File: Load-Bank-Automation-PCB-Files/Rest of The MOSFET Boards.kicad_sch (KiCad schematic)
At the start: 17 parts, among them J25 Conn_02x03_Counter_Clockwise, J27 PHNX_CONN_1017521, Q4 GSGN0648, U11 IRS10752LPBF, U9 ACS711xLCTR-25AB

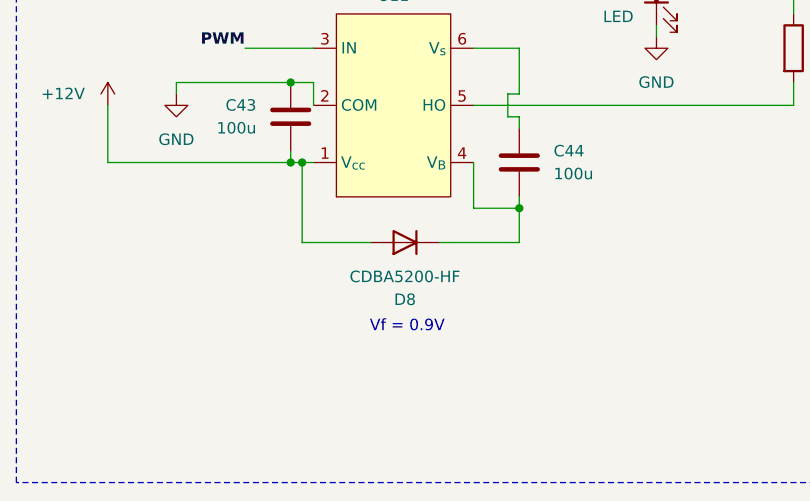
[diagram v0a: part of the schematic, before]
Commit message: Schematic for revision
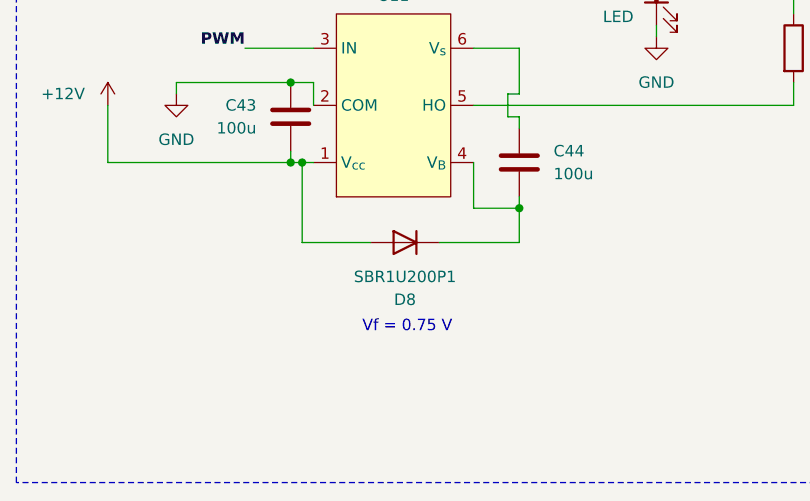
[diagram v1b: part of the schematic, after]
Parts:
- D8: value CDBA5200-HF -> SBR1U200P1; footprint Diode_SMD:D_SMA -> Diode_SMD:D_PowerDI-123
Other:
- note added: "Vf = 0.75 V"
- note removed: "Vf = 0.9V"
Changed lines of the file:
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@@
 		)
 	)
-	(text "Vf = 0.9V\n"
+	(text "Vf = 0.75 V\n"
 		(exclude_from_sim no)
 		(at 76.454 144.018 0)
@@
 	)
 	(symbol
+		(lib_id "Device:D")
+		(at 76.2 134.62 0)
+		(mirror y)
+		(unit 1)
+		(exclude_from_sim no)
+		(in_bom yes)
+		(on_board yes)
+		(dnp no)
+		(property "Reference" "D8"
+			(at 76.2 140.97 0)
+			(effects
+				(font
+					(size 1.27 1.27)
+				)
+			)
+		)
+		(property "Value" "SBR1U200P1"
+			(at 76.2 138.43 0)
+			(effects
+				(font
+					(size 1.27 1.27)
+				)
+			)
+		)
+		(property "Footprint" "Diode_SMD:D_PowerDI-123"
+			(at 76.2 134.62 0)
+			(effects
+				(font
+					(size 1.27 1.27)
+				)
+				(hide yes)
+			)
+		)
+		(property "Datasheet" "https://www.digikey.ca/en/products/detail/diodes-incorporated/SBR1U200P1-7/2414250"
+			(at 76.2 134.62 0)
+			(effects
+				(font
+					(size 1.27 1.27)
+				)
+				(hide yes)
+			)
+		)
+		(property "Description" "Diode"
+			(at 76.2 134.62 0)
+			(effects
+				(font
+					(size 1.27 1.27)
+				)
+				(hide yes)
+			)
+		)
+		(property "Sim.Device" "D"
+			(at 76.2 134.62 0)
+			(effects
+				(font
+					(size 1.27 1.27)
+				)
+				(hide yes)
+			)
+		)
+		(property "Sim.Pins" "1=K 2=A"
+			(at 76.2 134.62 0)
+			(effects
+				(font
+					(size 1.27 1.27)
+				)
+				(hide yes)
+			)
+		)
+		(pin "1"
+		)
+		(pin "2"
+		)
+		(instances
+			(project "Main Board"
+				(path "/c82c4769-33eb-46b7-8d07-39045014a3da/705e8481-c510-4db4-b00b-95a36c7dbdfb/1a67e662-c793-4736-b25e-544e5ea2a7f2"
+					(reference "D15")
+					(unit 1)
+				)
+				(path "/c82c4769-33eb-46b7-8d07-39045014a3da/705e8481-c510-4db4-b00b-95a36c7dbdfb/2277d187-c9b9-4e91-9f4d-91649daa1e71"
+					(reference "D25")
+					(unit 1)
+				)
+				(path "/c82c4769-33eb-46b7-8d07-39045014a3da/705e8481-c510-4db4-b00b-95a36c7dbdfb/227a110c-2de7-41e3-bc6f-746bf0261260"
+					(reference "D35")
+					(unit 1)
+				)
+				(path "/c82c4769-33eb-46b7-8d07-39045014a3da/705e8481-c510-4db4-b00b-95a36c7dbdfb/2c46a025-4a74-4b20-ae58-c6210c66e001"
+					(reference "D17")
+					(unit 1)
+				)
+				(path "/c82c4769-33eb-46b7-8d07-39045014a3da/705e8481-c510-4db4-b00b-95a36c7dbdfb/2e468d94-c9dd-45e8-83a4-34bc7627c87c"
+					(reference "D27")
+					(unit 1)
+				)
+				(path "/c82c4769-33eb-46b7-8d07-39045014a3da/705e8481-c510-4db4-b00b-95a36c7dbdfb/2f2c4eba-188b-4847-ac86-18b67317f14e"
+					(reference "D45")
+					(unit 1)
+				)
+				(path "/c82c4769-33eb-46b7-8d07-39045014a3da/705e8481-c510-4db4-b00b-95a36c7dbdfb/40b8ca81-553e-43de-ab2c-4f0caaabbcda"
+					(reference "D29")
+					(unit 1)
+				)
+				(path "/c82c4769-33eb-46b7-8d07-39045014a3da/705e8481-c510-4db4-b00b-95a36c7dbdfb/651d167a-11cf-47b6-a853-494d457f1bf4"
+					(reference "D21")
+					(unit 1)
+				)
+				(path "/c82c4769-33eb-46b7-8d07-39045014a3da/705e8481-c510-4db4-b00b-95a36c7dbdfb/6716ac13-3d47-413f-831f-be548b60f086"
+					(reference "D31")
+					(unit 1)
+				)
+				(path "/c82c4769-33eb-46b7-8d07-39045014a3da/705e8481-c510-4db4-b00b-95a36c7dbdfb/6bd58e0a-6e41-4d56-bd27-95eaa909d6f3"
+					(reference "D9")
+					(unit 1)
+				)
+				(path "/c82c4769-33eb-46b7-8d07-39045014a3da/705e8481-c510-4db4-b00b-95a36c7dbdfb/718b9ca6-7845-4b51-9b25-438e862042ea"
+					(reference "D8")
+					(unit 1)
+				)
+				(path "/c82c4769-33eb-46b7-8d07-39045014a3da/705e8481-c510-4db4-b00b-95a36c7dbdfb/8a426fe4-a42e-4f9e-af4e-eefac09b5ace"
+					(reference "D13")
+					(unit 1)
+				)
+				(path "/c82c4769-33eb-46b7-8d07-39045014a3da/705e8481-c510-4db4-b00b-95a36c7dbdfb/a9eaf66a-4f17-436c-8b91-843863372aaa"
+					(reference "D39")
+					(unit 1)
+				)
+				(path "/c82c4769-33eb-46b7-8d07-39045014a3da/705e8481-c510-4db4-b00b-95a36c7dbdfb/acf337b6-d238-4bef-aec6-ad93ba0b65cb"
+					(reference "D41")
+					(unit 1)
+				)
+				(path "/c82c4769-33eb-46b7-8d07-39045014a3da/705e8481-c510-4db4-b00b-95a36c7dbdfb/b8d87939-45d6-4d12-a59a-c885e34d5f0f"
+					(reference "D33")
+					(unit 1)
+				)
+				(path "/c82c4769-33eb-46b7-8d07-39045014a3da/705e8481-c510-4db4-b00b-95a36c7dbdfb/c491ae4d-a266-4cb1-ba09-71771eb863dc"
+					(reference "D43")
+					(unit 1)
+				)
+				(path "/c82c4769-33eb-46b7-8d07-39045014a3da/705e8481-c510-4db4-b00b-95a36c7dbdfb/c95f5c82-7dbb-483f-a16d-79c76a85d9aa"
+					(reference "D19")
+					(unit 1)
+				)
+				(path "/c82c4769-33eb-46b7-8d07-39045014a3da/705e8481-c510-4db4-b00b-95a36c7dbdfb/d9be4bd1-5e18-4dd0-8ec5-1e017de4b199"
+					(reference "D23")
+					(unit 1)
+				)
+				(path "/c82c4769-33eb-46b7-8d07-39045014a3da/705e8481-c510-4db4-b00b-95a36c7dbdfb/e74bb674-503c-4174-a688-cb850900d576"
+					(reference "D37")
+					(unit 1)
+				)
+			)
+		)
+	)
+	(symbol
 		(lib_id "Sensor_Current:ACS711xLCTR-25AB")
 		(at 171.45 72.39 270)
@@
 					(unit 1)
 				)
-			)
-		)
-	)
-	(symbol
-		(lib_id "Device:D")
-		(at 76.2 134.62 180)
-		(unit 1)
-		(exclude_from_sim no)
-		(in_bom yes)
-		(on_board yes)
-		(dnp no)
-		(property "Reference" "D8"
-			(at 76.2 140.97 0)
-			(effects
-				(font
-					(size 1.27 1.27)
-				)
-			)
-		)
-		(property "Value" "CDBA5200-HF"
-			(at 76.2 138.43 0)
-			(effects
-				(font
-					(size 1.27 1.27)
-				)
-			)
-		)
-		(property "Footprint" "Diode_SMD:D_SMA"
-			(at 76.2 134.62 0)
-			(effects
-				(font
-					(size 1.27 1.27)
-				)
-				(hide yes)
-			)
-		)
-		(property "Datasheet" "https://mm.digikey.com/Volume0/opasdata/d220001/medias/docus/506/CDBA540-HF-CDBA5200-HF_RevC.pdf"
-			(at 76.2 134.62 0)
-			(effects
-				(font
-					(size 1.27 1.27)
-				)
-				(hide yes)
-			)
-		)
-		(property "Description" "Diode"
-			(at 76.2 134.62 0)
-			(effects
-				(font
-					(size 1.27 1.27)
-				)
-				(hide yes)
-			)
-		)
-		(property "Sim.Device" "D"
-			(at 76.2 134.62 0)
-			(effects
-				(font
-					(size 1.27 1.27)
-				)
-				(hide yes)
-			)
-		)
-		(property "Sim.Pins" "1=K 2=A"
-			(at 76.2 134.62 0)
-			(effects
-				(font
-					(size 1.27 1.27)
-				)
-				(hide yes)
-			)
-		)
-		(pin "1"
-		)
-		(pin "2"
-		)
-		(instances
-			(project "Main Board"
-				(path "/c82c4769-33eb-46b7-8d07-39045014a3da/705e8481-c510-4db4-b00b-95a36c7dbdfb/1a67e662-c793-4736-b25e-544e5ea2a7f2"
-					(reference "D15")
-					(unit 1)
-				)
-				(path "/c82c4769-33eb-46b7-8d07-39045014a3da/705e8481-c510-4db4-b00b-95a36c7dbdfb/2277d187-c9b9-4e91-9f4d-91649daa1e71"
-					(reference "D25")
-					(unit 1)
-				)
-				(path "/c82c4769-33eb-46b7-8d07-39045014a3da/705e8481-c510-4db4-b00b-95a36c7dbdfb/227a110c-2de7-41e3-bc6f-746bf0261260"
-					(reference "D35")
-					(unit 1)
-				)
-				(path "/c82c4769-33eb-46b7-8d07-39045014a3da/705e8481-c510-4db4-b00b-95a36c7dbdfb/2c46a025-4a74-4b20-ae58-c6210c66e001"
-					(reference "D17")
-					(unit 1)
-				)
-				(path "/c82c4769-33eb-46b7-8d07-39045014a3da/705e8481-c510-4db4-b00b-95a36c7dbdfb/2e468d94-c9dd-45e8-83a4-34bc7627c87c"
-					(reference "D27")
-					(unit 1)
-				)
-				(path "/c82c4769-33eb-46b7-8d07-39045014a3da/705e8481-c510-4db4-b00b-95a36c7dbdfb/2f2c4eba-188b-4847-ac86-18b67317f14e"
-					(reference "D45")
-					(unit 1)
-				)
-				(path "/c82c4769-33eb-46b7-8d07-39045014a3da/705e8481-c510-4db4-b00b-95a36c7dbdfb/40b8ca81-553e-43de-ab2c-4f0caaabbcda"
-					(reference "D29")
-					(unit 1)
-				)
-				(path "/c82c4769-33eb-46b7-8d07-39045014a3da/705e8481-c510-4db4-b00b-95a36c7dbdfb/651d167a-11cf-47b6-a853-494d457f1bf4"
-					(reference "D21")
-					(unit 1)
-				)
-				(path "/c82c4769-33eb-46b7-8d07-39045014a3da/705e8481-c510-4db4-b00b-95a36c7dbdfb/6716ac13-3d47-413f-831f-be548b60f086"
-					(reference "D31")
-					(unit 1)
-				)
-				(path "/c82c4769-33eb-46b7-8d07-39045014a3da/705e8481-c510-4db4-b00b-95a36c7dbdfb/6bd58e0a-6e41-4d56-bd27-95eaa909d6f3"
-					(reference "D9")
-					(unit 1)
-				)
-				(path "/c82c4769-33eb-46b7-8d07-39045014a3da/705e8481-c510-4db4-b00b-95a36c7dbdfb/718b9ca6-7845-4b51-9b25-438e862042ea"
-					(reference "D8")
-					(unit 1)
-				)
-				(path "/c82c4769-33eb-46b7-8d07-39045014a3da/705e8481-c510-4db4-b00b-95a36c7dbdfb/8a426fe4-a42e-4f9e-af4e-eefac09b5ace"
-					(reference "D13")
-					(unit 1)
-				)
-				(path "/c82c4769-33eb-46b7-8d07-39045014a3da/705e8481-c510-4db4-b00b-95a36c7dbdfb/a9eaf66a-4f17-436c-8b91-843863372aaa"
-					(reference "D39")
-					(unit 1)
-				)
-				(path "/c82c4769-33eb-46b7-8d07-39045014a3da/705e8481-c510-4db4-b00b-95a36c7dbdfb/acf337b6-d238-4bef-aec6-ad93ba0b65cb"
-					(reference "D41")
-					(unit 1)
-				)
-				(path "/c82c4769-33eb-46b7-8d07-39045014a3da/705e8481-c510-4db4-b00b-95a36c7dbdfb/b8d87939-45d6-4d12-a59a-c885e34d5f0f"
-					(reference "D33")
-					(unit 1)
-				)
-				(path "/c82c4769-33eb-46b7-8d07-39045014a3da/705e8481-c510-4db4-b00b-95a36c7dbdfb/c491ae4d-a266-4cb1-ba09-71771eb863dc"
-					(reference "D43")
-					(unit 1)
-				)
-				(path "/c82c4769-33eb-46b7-8d07-39045014a3da/705e8481-c510-4db4-b00b-95a36c7dbdfb/c95f5c82-7dbb-483f-a16d-79c76a85d9aa"
-					(reference "D19")
-					(unit 1)
-				)
-				(path "/c82c4769-33eb-46b7-8d07-39045014a3da/705e8481-c510-4db4-b00b-95a36c7dbdfb/d9be4bd1-5e18-4dd0-8ec5-1e017de4b199"
-					(reference "D23")
-					(unit 1)
-				)
-				(path "/c82c4769-33eb-46b7-8d07-39045014a3da/705e8481-c510-4db4-b00b-95a36c7dbdfb/e74bb674-503c-4174-a688-cb850900d576"
-					(reference "D37")
-					(unit 1)
-				)
